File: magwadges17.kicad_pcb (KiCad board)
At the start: 2 copper layers, 156 x 89.8 mm, 44 parts, among them J1 PGM, J2 JACK_2P, U1 ATTINY861A-SU

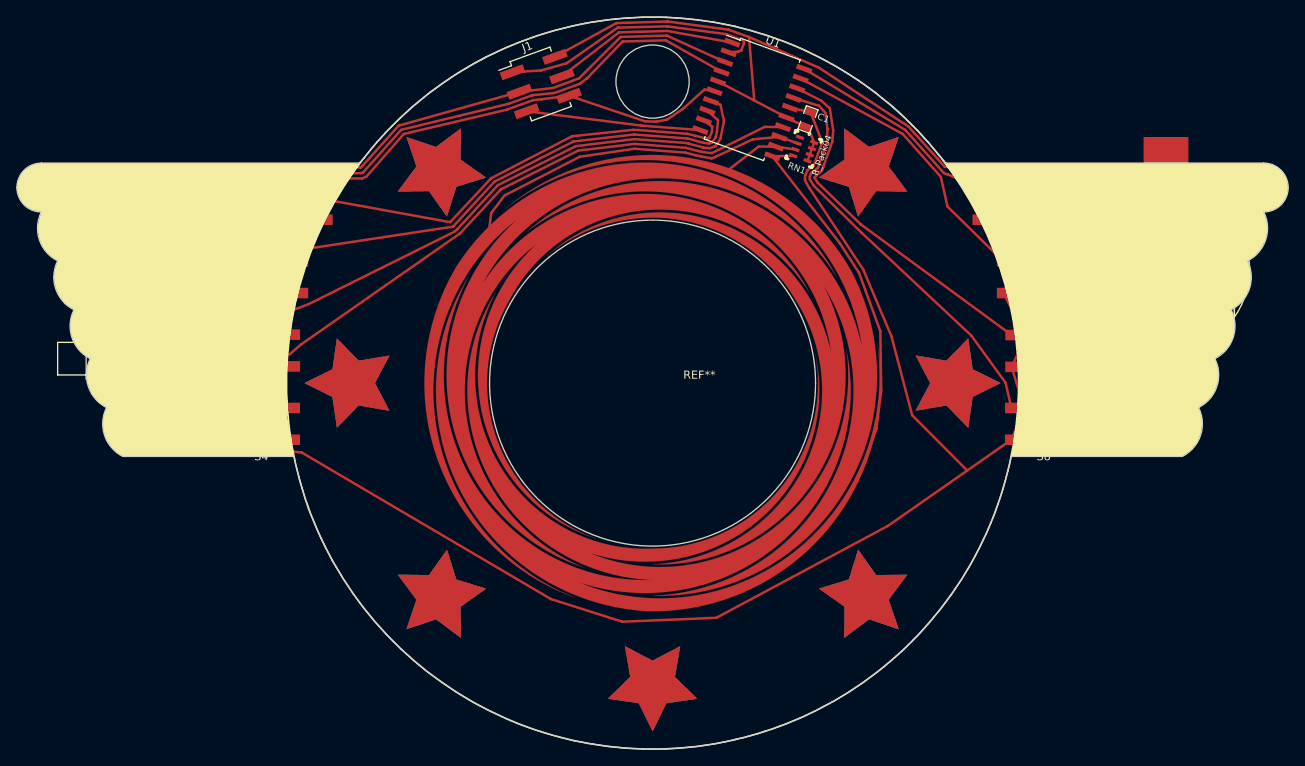
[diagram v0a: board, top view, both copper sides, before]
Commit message: Update wadges
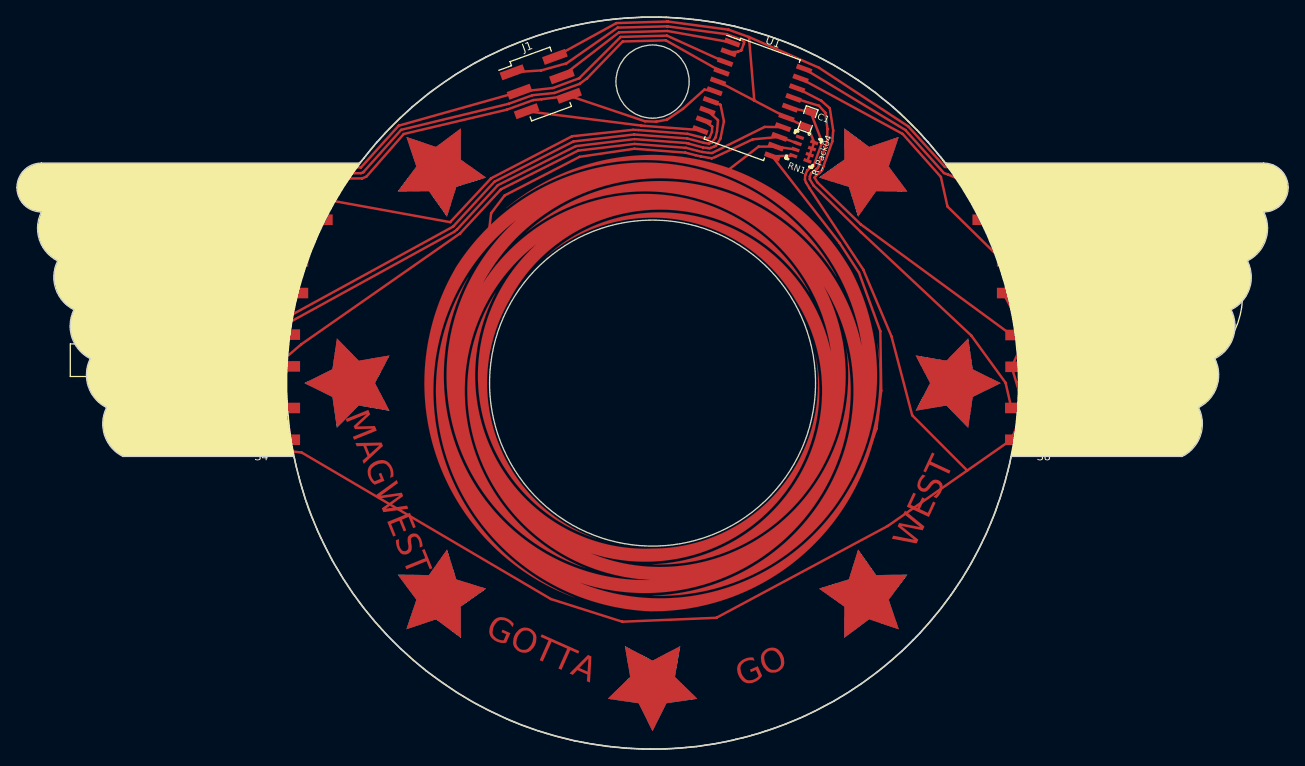
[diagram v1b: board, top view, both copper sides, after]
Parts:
- moved BT1 3.30 mm to (212.1, 89.2)
- moved J2 1.56 mm to (83.5, 97.2)
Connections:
- J1 pad 3: Net-(J1-Pad3) -> SW_F
- LS1 pad 2: Net-(J1-Pad3) -> Net-(LS1-Pad2)
- U1 pad 3: Net-(J1-Pad3) -> SW_F
- U1 pad 4: Net-(J2-Pad2) -> SW_G
- U1 pad 7: SW_F -> Net-(LS1-Pad2)
- U1 pad 8: SW_G -> Net-(J2-Pad2)
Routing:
- net Net-(LS1-Pad2): track 0.00 -> 110.1 mm
- net Net-(J1-Pad3): track 85.9 -> 0.00 mm
- net GND: track 323.4 -> 371.3 mm
- net SW_F: track 72.9 -> 85.7 mm
- net SW_G: track 67.0 -> 75.3 mm
- net Net-(J2-Pad2): track 99.5 -> 106.3 mm
- net VCC: track 127.7 -> 134.3 mm
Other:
- board text added: "GO"
- board text added: "GOTTA"
- board text added: "MAGWEST"
- board text added: "WEST"
